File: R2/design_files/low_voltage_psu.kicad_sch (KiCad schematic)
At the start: 9 parts, among them U13 PUMH10,115, U9 AP61100Z6

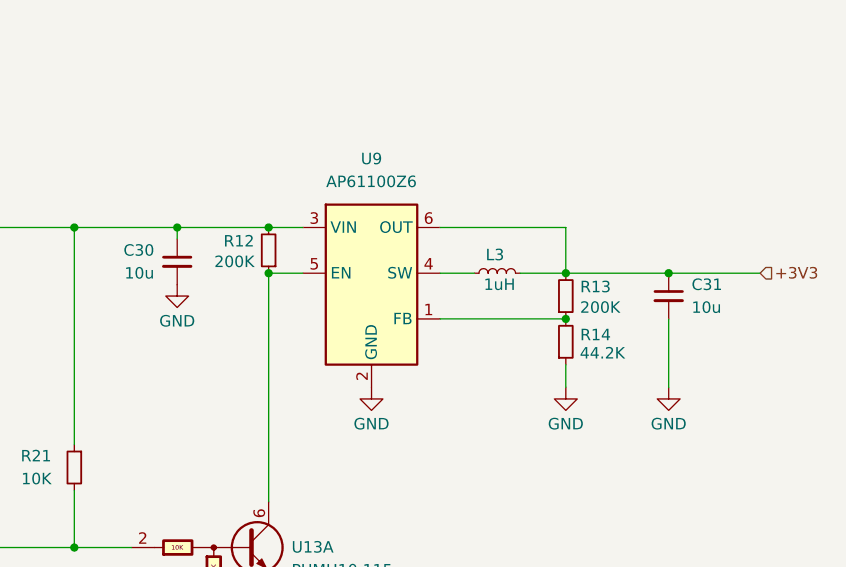
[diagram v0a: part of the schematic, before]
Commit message: Refactor code structure for improved readability and maintainability
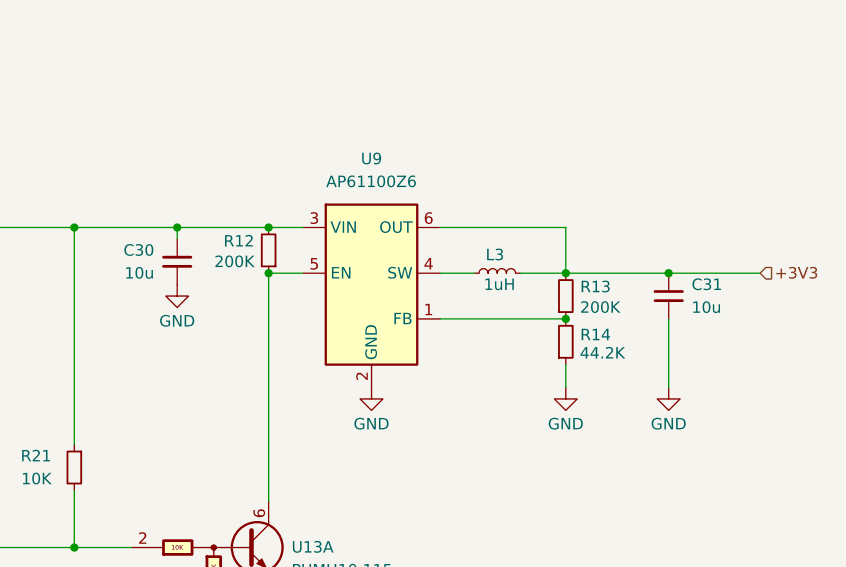
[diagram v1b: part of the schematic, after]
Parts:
- L3: footprint My Footprints:L_0806_2016Metric_TAIYO_YUDEN_SMD -> My_Footprints:L_0806_2016Metric_TAIYO_YUDEN_SMD
- U9: symbol My Libraries:AP61100Z6 -> My_Libraries:AP61100Z6

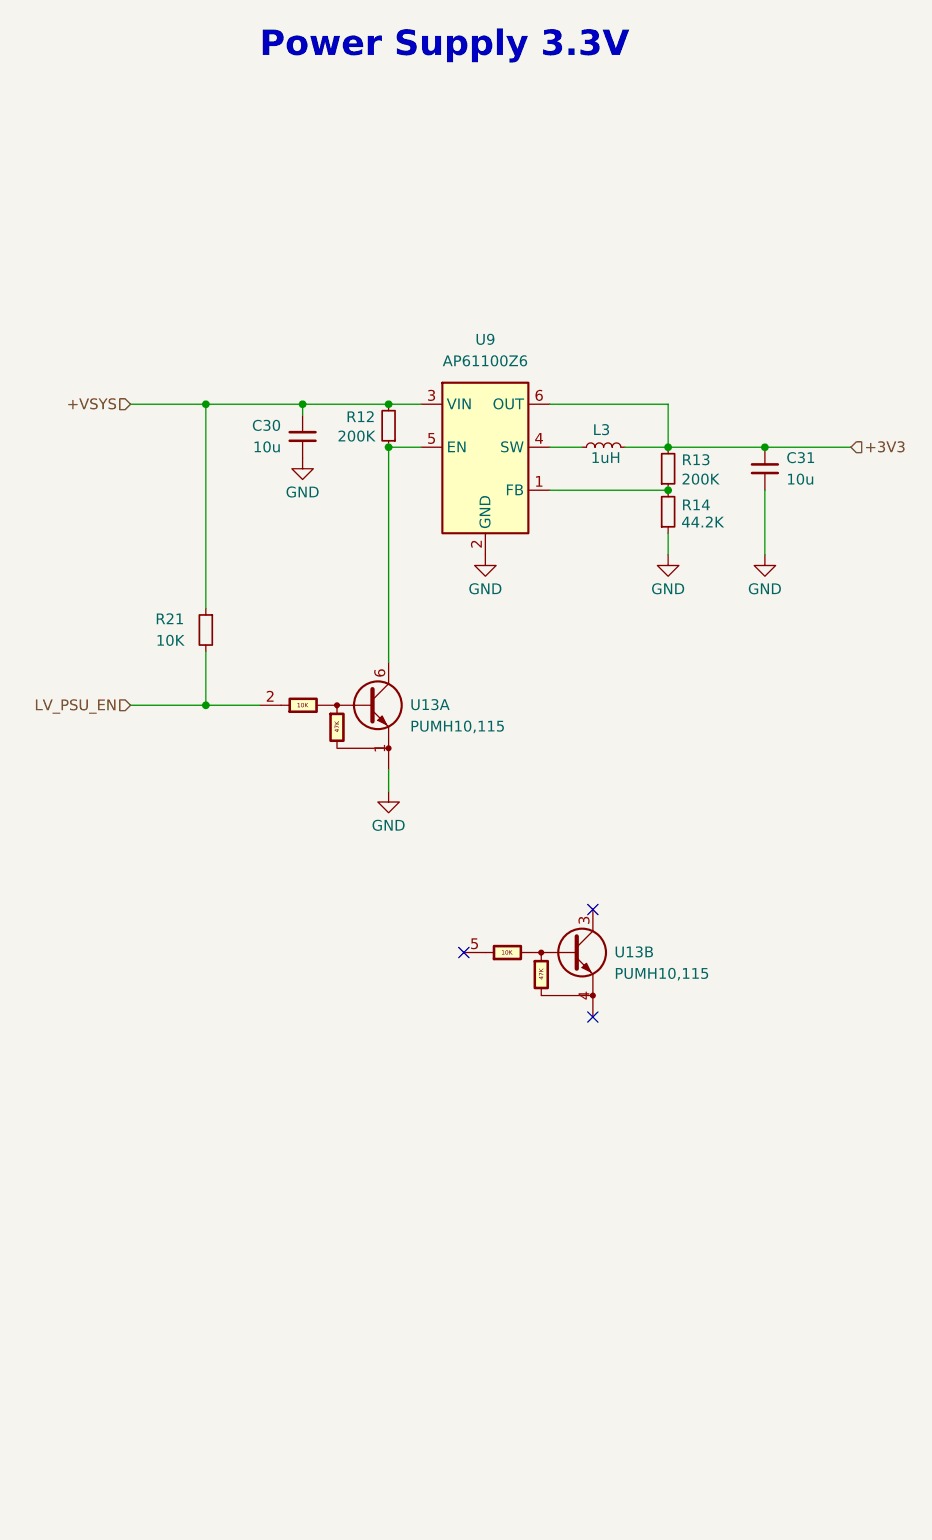
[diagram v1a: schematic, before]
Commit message: Refactor code structure for improved readability and maintainability
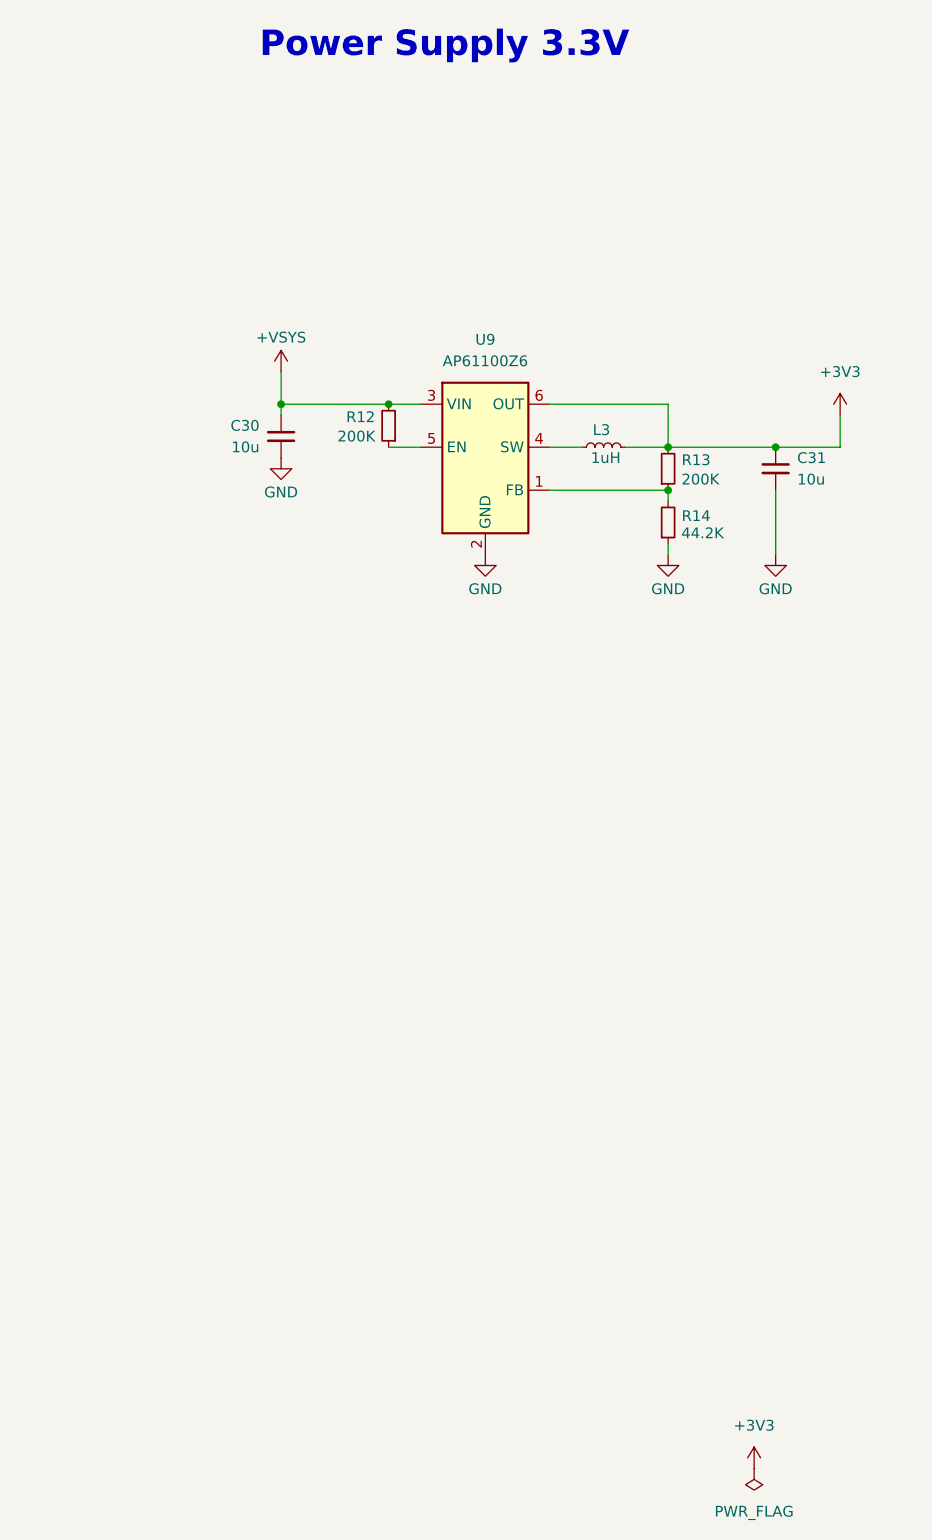
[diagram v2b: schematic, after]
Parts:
- removed R21: 10K, Resistor_SMD:R_0402_1005Metric, symbol Device:R_Small
- removed U13: PUMH10,115, Package_TO_SOT_SMD:SOT-363_SC-70-6, symbol My_Libraries:PUMH10,115
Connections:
- no-connect marks 3 -> 0
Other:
- moved on the sheet: C30, C31, R14
